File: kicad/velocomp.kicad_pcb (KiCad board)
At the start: 2 copper layers, 45 x 30 mm, 31 parts, among them IC1 STM8S003F3P, J1 USB_B, J2 h2_g, J3 prg, J4 h2, J5 kn1, J6 kn1, Q1 2N7002, SW1 SW_PUSH, SW2 Herkon, U1 BK3231, U2 TP4056, Y1 8Mgh

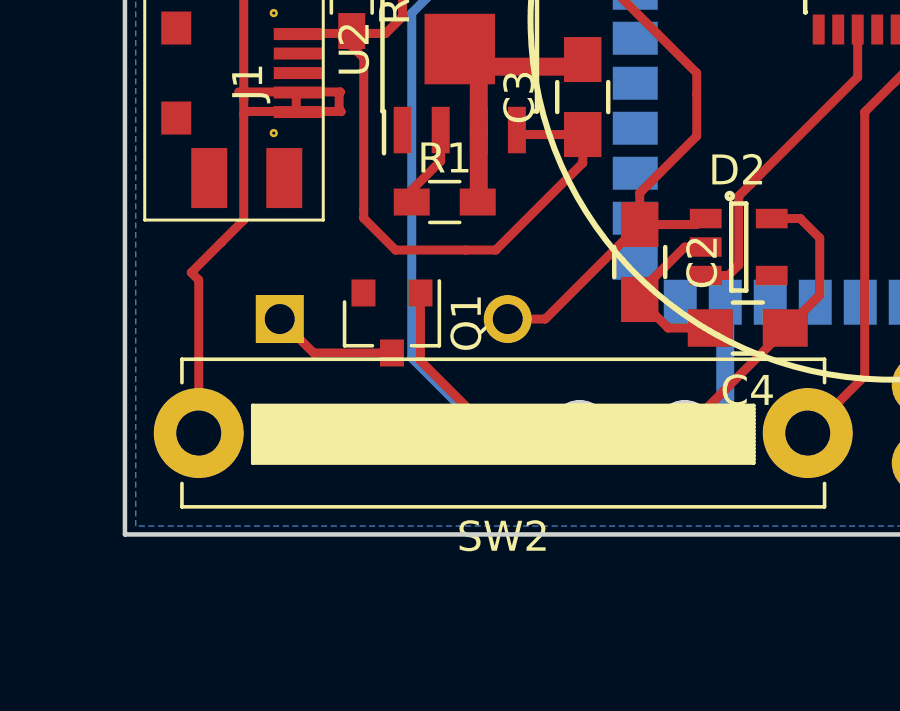
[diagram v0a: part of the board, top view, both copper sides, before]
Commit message: start
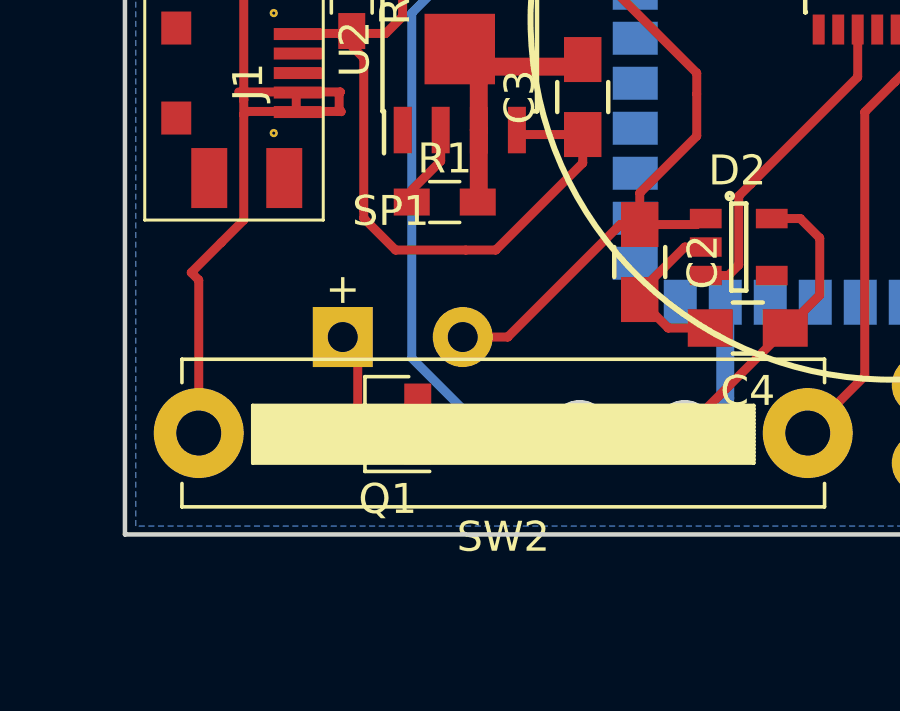
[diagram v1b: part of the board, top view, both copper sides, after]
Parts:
- C2, C4: value 1u -> 1uf
- SP1: footprint Buzzers_Beepers:MagneticBuzzer_ProSignal_ABI-009-RC -> mylibpcb:hc0903a; moved to F.Cu
- moved Q1 3.37 mm to (78.8, 76.3), turned to 180 degrees
- moved SP1 2.18 mm to (77.3, 73.4)
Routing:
- net /spk: track 51.4 -> 48.4 mm
- net VDD: track 47.9 -> 49.6 mm
- net Net-(Q1-Pad3): track 4.48 -> 3.39 mm
